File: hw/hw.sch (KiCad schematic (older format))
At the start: 12 parts, among them U1 74LS299, U2 74LS138, U3 Z80CPU, U4 74LS161, U5 CY7C199, U6 74LS107, X1 CXO_DIP8

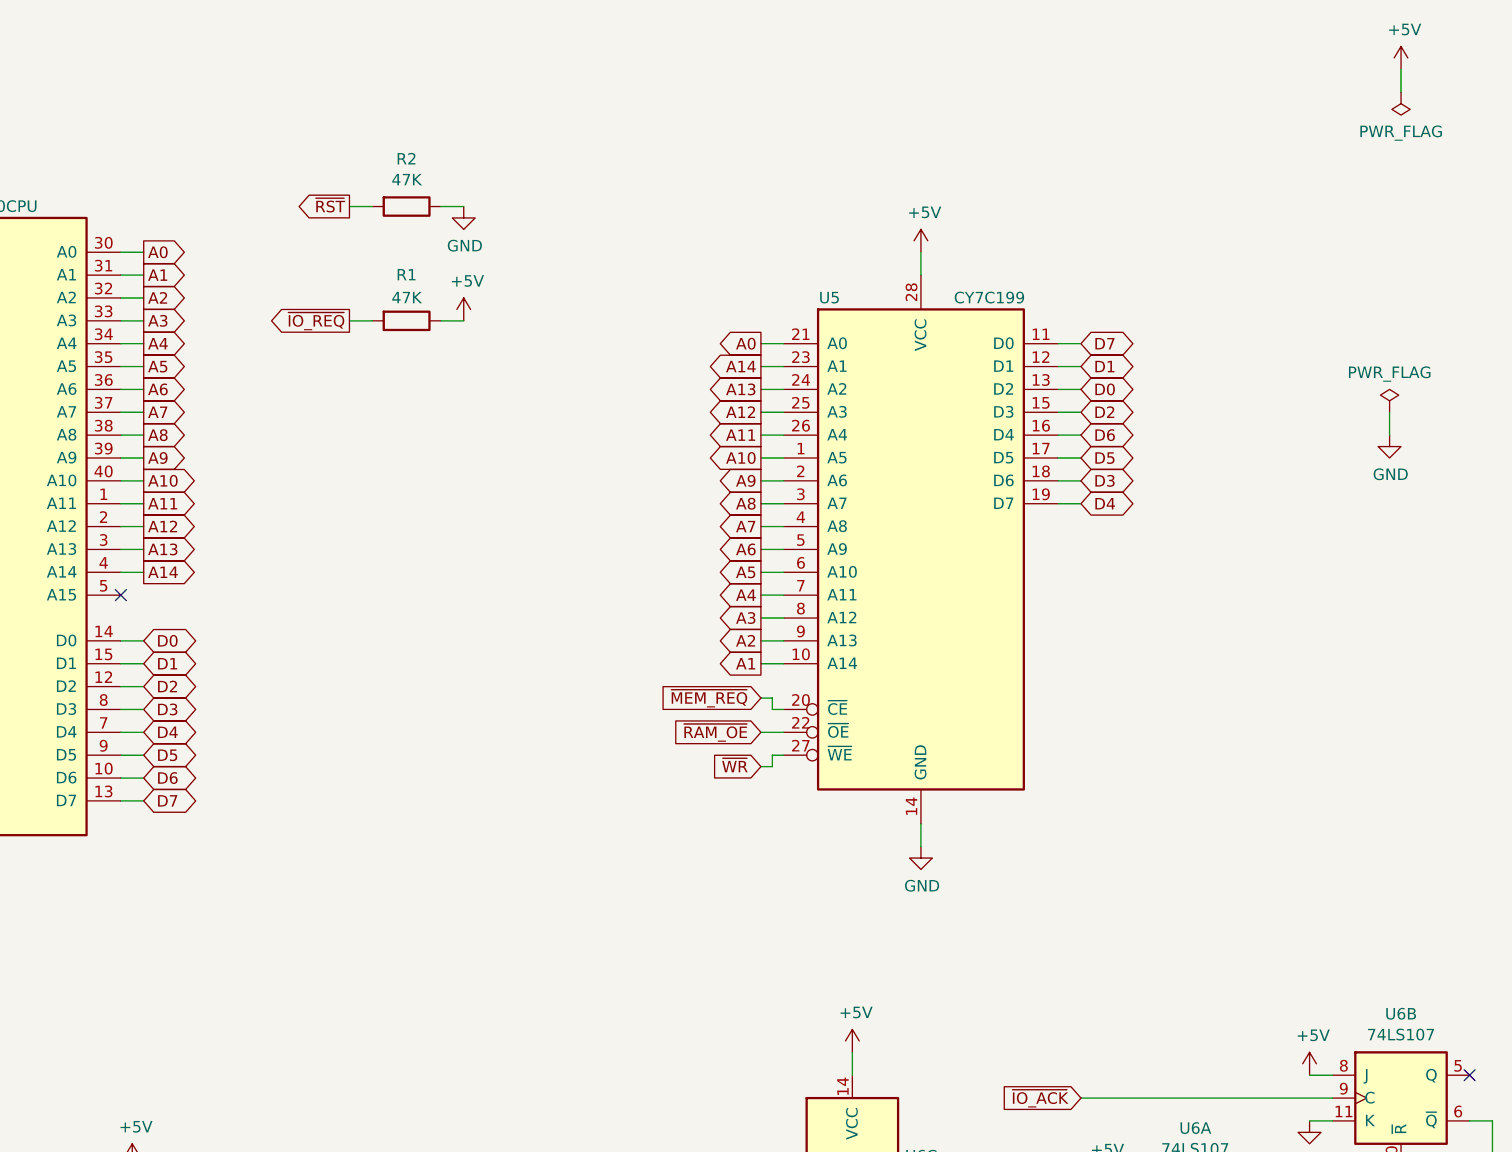
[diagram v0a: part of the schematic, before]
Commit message: add output port
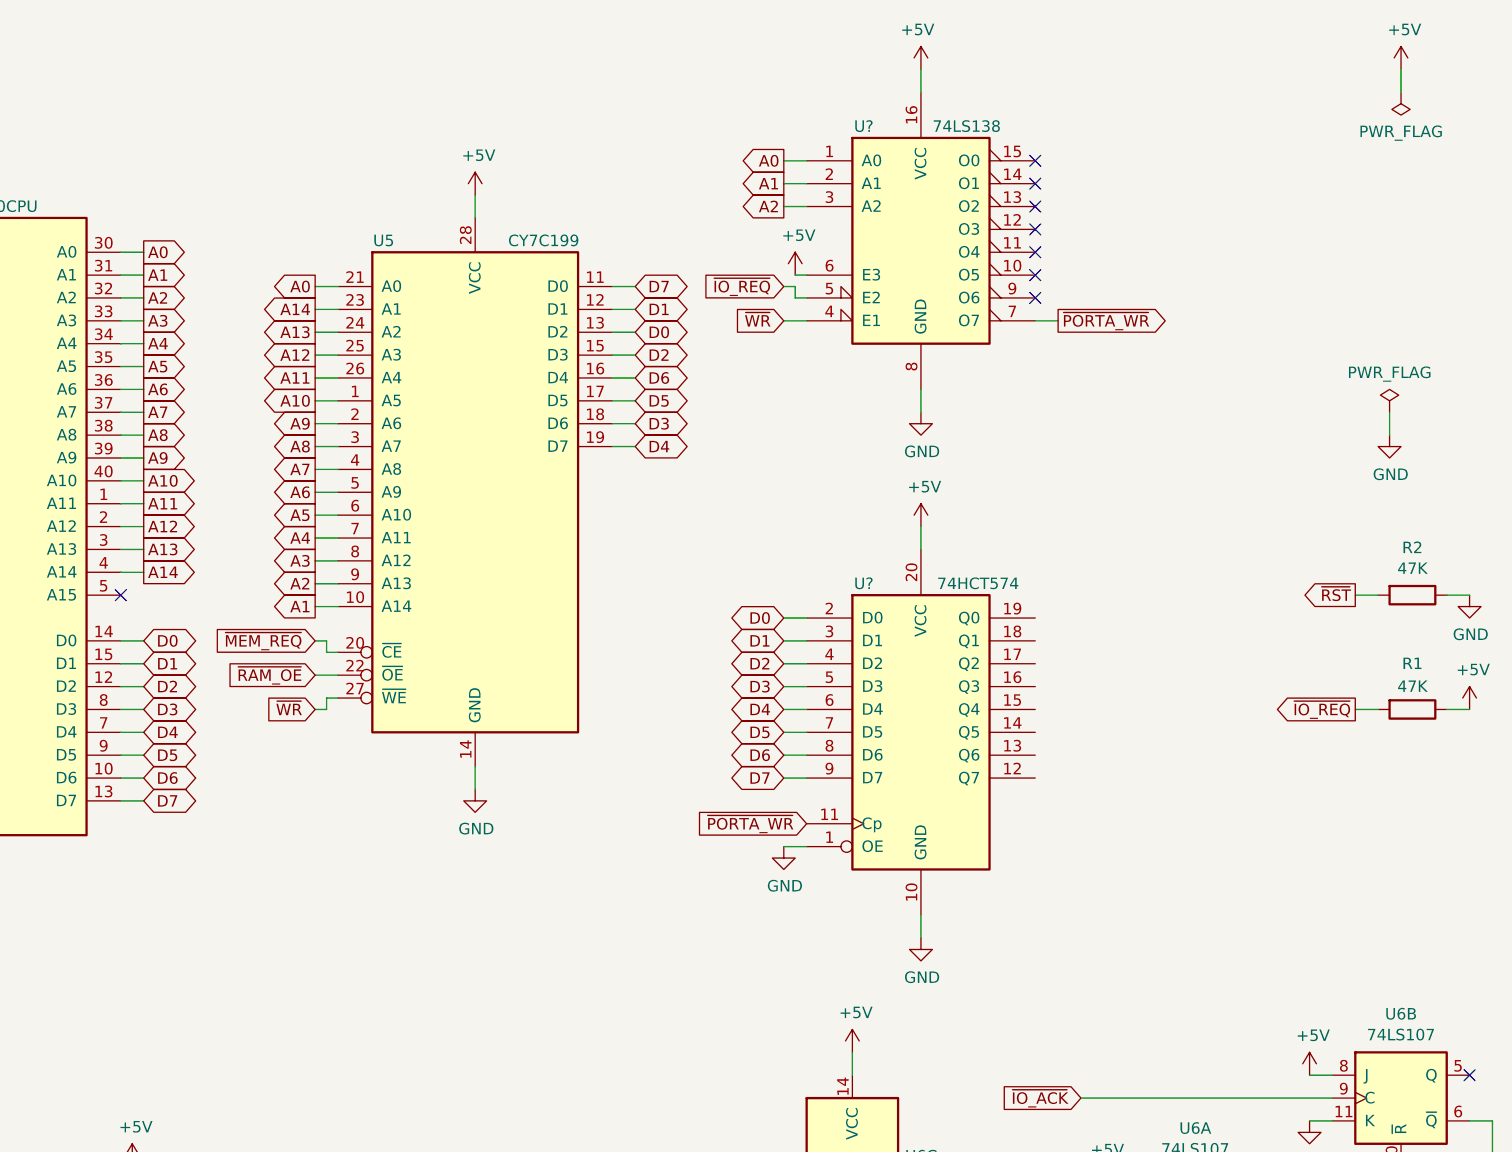
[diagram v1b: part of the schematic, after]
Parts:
- added U?: 74LS138, symbol 74xx:74LS138
- added U?: 74HCT574, symbol 74xx:74HCT574
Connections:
- net +5V: now also U?.16 (VCC), U?.20 (VCC), U?.6 (E3)
- net A0: now also U?.1 (A0)
- net A1: now also U?.2 (A1)
- net A2: now also U?.3 (A2)
- net D0: now also U?.2 (D0)
- net D1: now also U?.3 (D1)
- net D2: now also U?.4 (D2)
- net D3: now also U?.5 (D3)
- net D4: now also U?.6 (D4)
- net D5: now also U?.7 (D5)
- net D6: now also U?.8 (D6)
- net D7: now also U?.9 (D7)
- net GND: now also U?.1 (OE), U?.10 (GND), U?.8 (GND)
- net ~IO_REQ: now also U?.5 (E2)
- net ~WR: now also U?.4 (E1)
- new net ~PORTA_WR: U?.11 (Cp), U?.7 (O7)
- no-connect marks 32 -> 39
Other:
- moved on the sheet: R1, R2, U5
